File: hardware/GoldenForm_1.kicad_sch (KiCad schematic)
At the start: 29 parts, among them IC1 UVLO, J1 SD_Socket, J2 USB_C_Receptacle_USB2.0_14P, J3 Conn_01x04_Pin, M3 MountingHole x 4, SW1 BOOT, SW2 RESET, U1 Buck_Boost, U2 BNO055, U4 ESP32-S3-WROOM-1

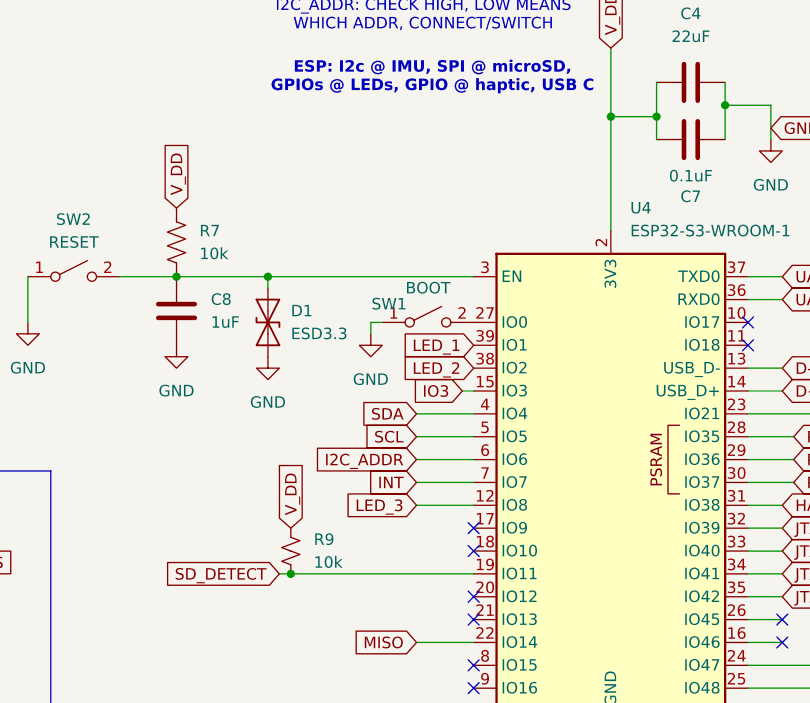
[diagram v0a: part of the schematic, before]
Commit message: wip
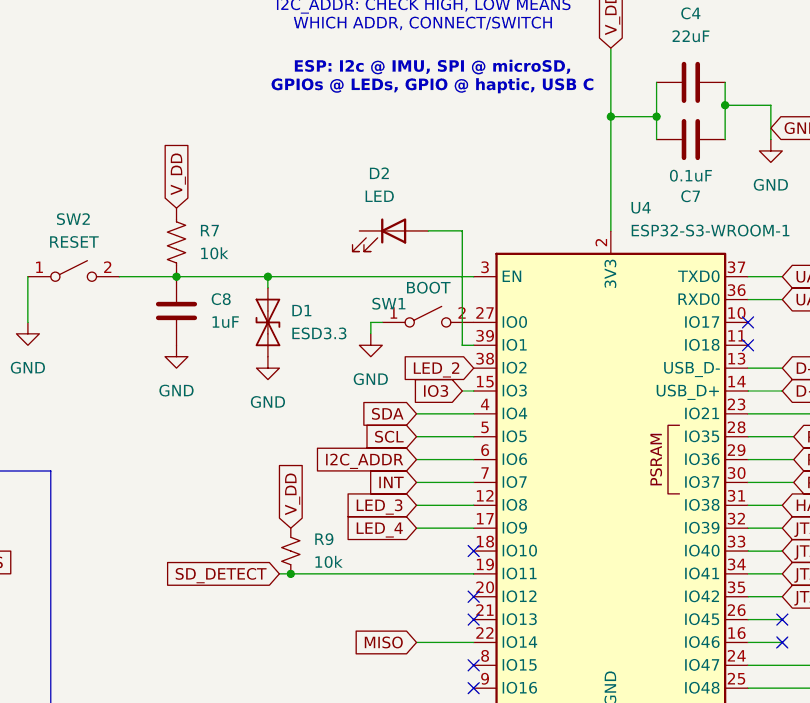
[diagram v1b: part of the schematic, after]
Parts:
- added D2: LED, symbol Device:LED
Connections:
- net LED_4: now reaches U4.17 (IO9)
- net LED_1: no longer names the net of U4.39 (IO1)
- net LED_1: now also D2.2 (A)
- no-connect marks 15 -> 14
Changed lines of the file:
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@@
 	)
 	(no_connect
-		(at 128.27 77.47)
-	)
-	(no_connect
 		(at 128.27 87.63)
 	)
@@
 	(wire
 		(pts
+			(xy 123.19 44.45) (xy 127 44.45)
+		)
+		(stroke
+			(width 0)
+			(type default)
+		)
+	)
+	(wire
+		(pts
 			(xy 45.72 99.06) (xy 50.8 99.06)
 		)
@@
 	(wire
 		(pts
+			(xy 127 44.45) (xy 127 57.15)
+		)
+		(stroke
+			(width 0)
+			(type default)
+		)
+	)
+	(wire
+		(pts
 			(xy 139.7 100.33) (xy 143.51 100.33)
 		)
@@
 	(wire
 		(pts
+			(xy 127 57.15) (xy 128.27 57.15)
+		)
+		(stroke
+			(width 0)
+			(type default)
+		)
+	)
+	(wire
+		(pts
 			(xy 105.41 49.53) (xy 128.27 49.53)
 		)
@@
 	(wire
 		(pts
+			(xy 121.92 77.47) (xy 128.27 77.47)
+		)
+		(stroke
+			(width 0)
+			(type default)
+		)
+	)
+	(wire
+		(pts
 			(xy 101.6 151.13) (xy 100.33 151.13)
 		)
@@
 		)
 	)
+	(global_label "LED_4"
+		(shape input)
+		(at 121.92 77.47 180)
+		(fields_autoplaced yes)
+		(effects
+			(font
+				(size 1.27 1.27)
+			)
+			(justify right)
+		)
+		(property "Intersheetrefs" "${INTERSHEET_REFS}"
+			(at 113.3106 77.47 0)
+			(effects
+				(font
+					(size 1.27 1.27)
+				)
+				(justify right)
+				(hide yes)
+			)
+		)
+	)
 	(global_label "UART_RX"
 		(shape input)
@@
 		)
 	)
-	(global_label "LED_1"
-		(shape input)
-		(at 128.27 57.15 180)
-		(fields_autoplaced yes)
-		(effects
-			(font
-				(size 1.27 1.27)
-			)
-			(justify right)
-		)
-		(property "Intersheetrefs" "${INTERSHEET_REFS}"
-			(at 119.6606 57.15 0)
-			(effects
-				(font
-					(size 1.27 1.27)
-				)
-				(justify right)
-				(hide yes)
-			)
-		)
-	)
 	(global_label "GND"
 		(shape input)
@@
 					(unit 1)
 				)
+			)
+		)
+	)
+	(symbol
+		(lib_id "Device:LED")
+		(at 119.38 44.45 0)
+		(unit 1)
+		(exclude_from_sim no)
+		(in_bom yes)
+		(on_board yes)
+		(dnp no)
+		(fields_autoplaced yes)
+		(property "Reference" "D2"
+			(at 117.7925 38.1 0)
+			(effects
+				(font
+					(size 1.27 1.27)
+				)
+			)
+		)
+		(property "Value" "LED"
+			(at 117.7925 40.64 0)
+			(effects
+				(font
+					(size 1.27 1.27)
+				)
+			)
+		)
+		(property "Footprint" ""
+			(at 119.38 44.45 0)
+			(effects
+				(font
+					(size 1.27 1.27)
+				)
+				(hide yes)
+			)
+		)
+		(property "Datasheet" "~"
+			(at 119.38 44.45 0)
+			(effects
+				(font
+					(size 1.27 1.27)
+				)
+				(hide yes)
+			)
+		)
+		(property "Description" "Light emitting diode"
+			(at 119.38 44.45 0)
+			(effects
+				(font
+					(size 1.27 1.27)
+				)
+				(hide yes)
+			)
+		)
+		(property "Sim.Pins" "1=K 2=A"
+			(at 119.38 44.45 0)
+			(effects
+				(font
+					(size 1.27 1.27)
+				)
+				(hide yes)
+			)
+		)
+		(pin "1"
+		)
+		(pin "2"
+		)
+		(instances
+			(project "GoldenForm_1"
+				(path "/64cfd788-f968-4e49-826d-6322743ab44f"
+					(reference "D2")
+					(unit 1)
+				)
